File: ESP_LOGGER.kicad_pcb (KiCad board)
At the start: 2 copper layers, 75.6 x 62.2 mm, 29 parts, among them SW1 SW_Push, SW2 SW_Push, U1 AZ1086_SOT223

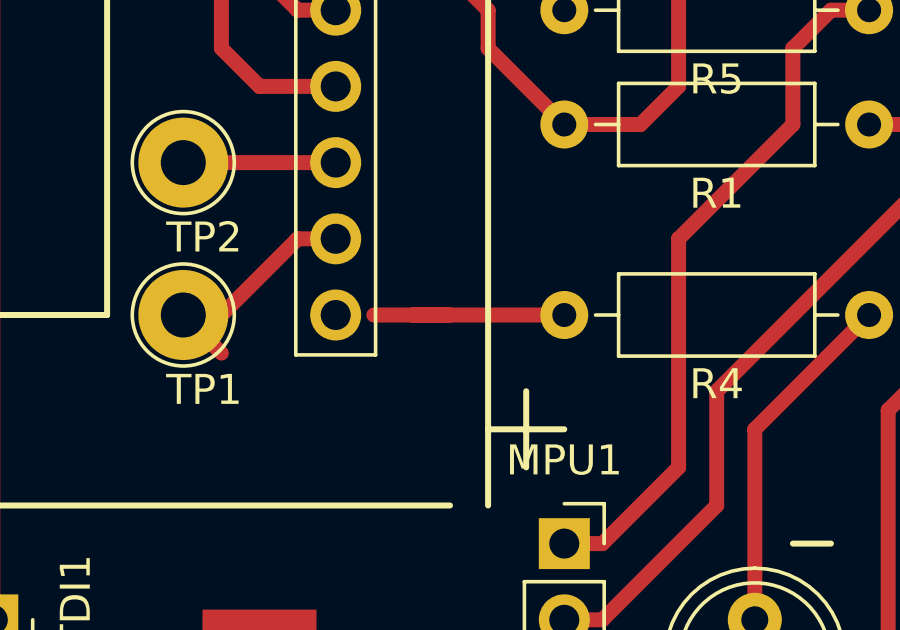
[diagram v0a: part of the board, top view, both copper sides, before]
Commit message: bugfix
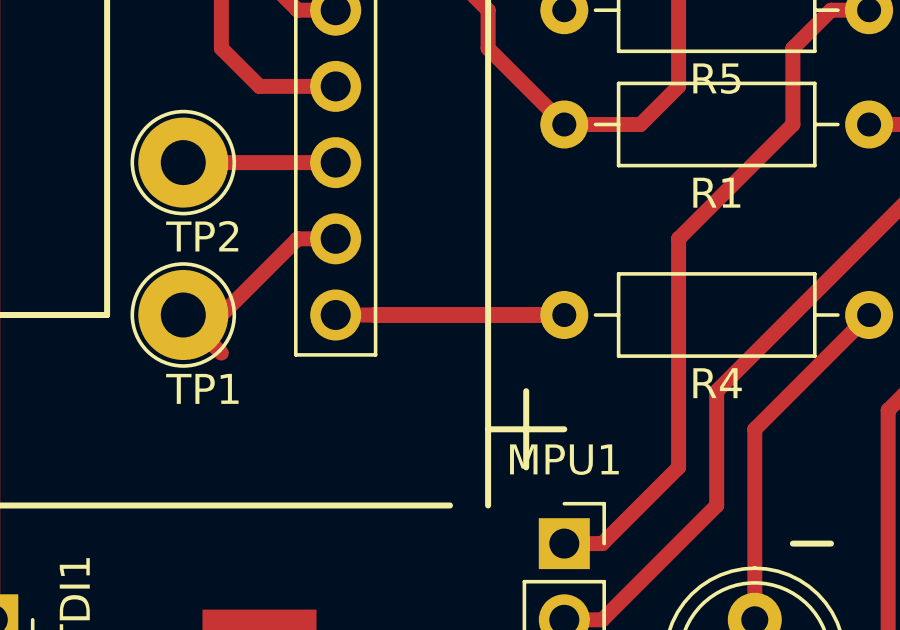
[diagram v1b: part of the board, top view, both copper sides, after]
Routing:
- net IO_LED: track 7.62 -> 15.2 mm
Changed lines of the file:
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@@
     (thickness 1.6)
     (drawings 30)
-    (tracks 160)
+    (tracks 162)
     (zones 0)
     (modules 29)
@@
   (segment (start 153.67 73.66) (end 158.75 73.66) (width 0.5) (layer F.Cu) (net 21) (status 30))
   (segment (start 152.4 73.66) (end 154.94 73.66) (width 0.5) (layer F.Cu) (net 21))
+  (segment (start 151.13 73.66) (end 152.4 73.66) (width 0.5) (layer F.Cu) (net 21))
+  (segment (start 152.4 73.66) (end 158.75 73.66) (width 0.5) (layer F.Cu) (net 21))
   (segment (start 179.07 58.42) (end 179.07 64.77) (width 0.5) (layer F.Cu) (net 22) (status 30))
   (segment (start 177.8 74.93) (end 179.07 74.93) (width 0.5) (layer F.Cu) (net 23) (status 20))
